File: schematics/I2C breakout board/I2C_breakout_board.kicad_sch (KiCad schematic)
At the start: 22 parts, among them J1 Conn_01x01_Pin, J10 Conn_01x01_Pin, J11 Conn_01x01_Pin, J12 Conn_01x01_Pin, J13 Conn_01x01_Pin, J14 Conn_01x01_Pin, J15 Conn_01x01_Pin, J16 Conn_01x01_Pin, J17 Conn_01x01_Pin, J2 Conn_01x01_Pin, J3 Conn_01x01_Pin, J4 Conn_01x01_Pin, J5 Conn_01x01_Pin, J6 Conn_01x01_Pin, J7 Conn_01x01_Pin, J8 Conn_01x01_Pin, J9 Conn_01x01_Pin, U1 ENS210-LQFM, U2 OPT4001DTSR

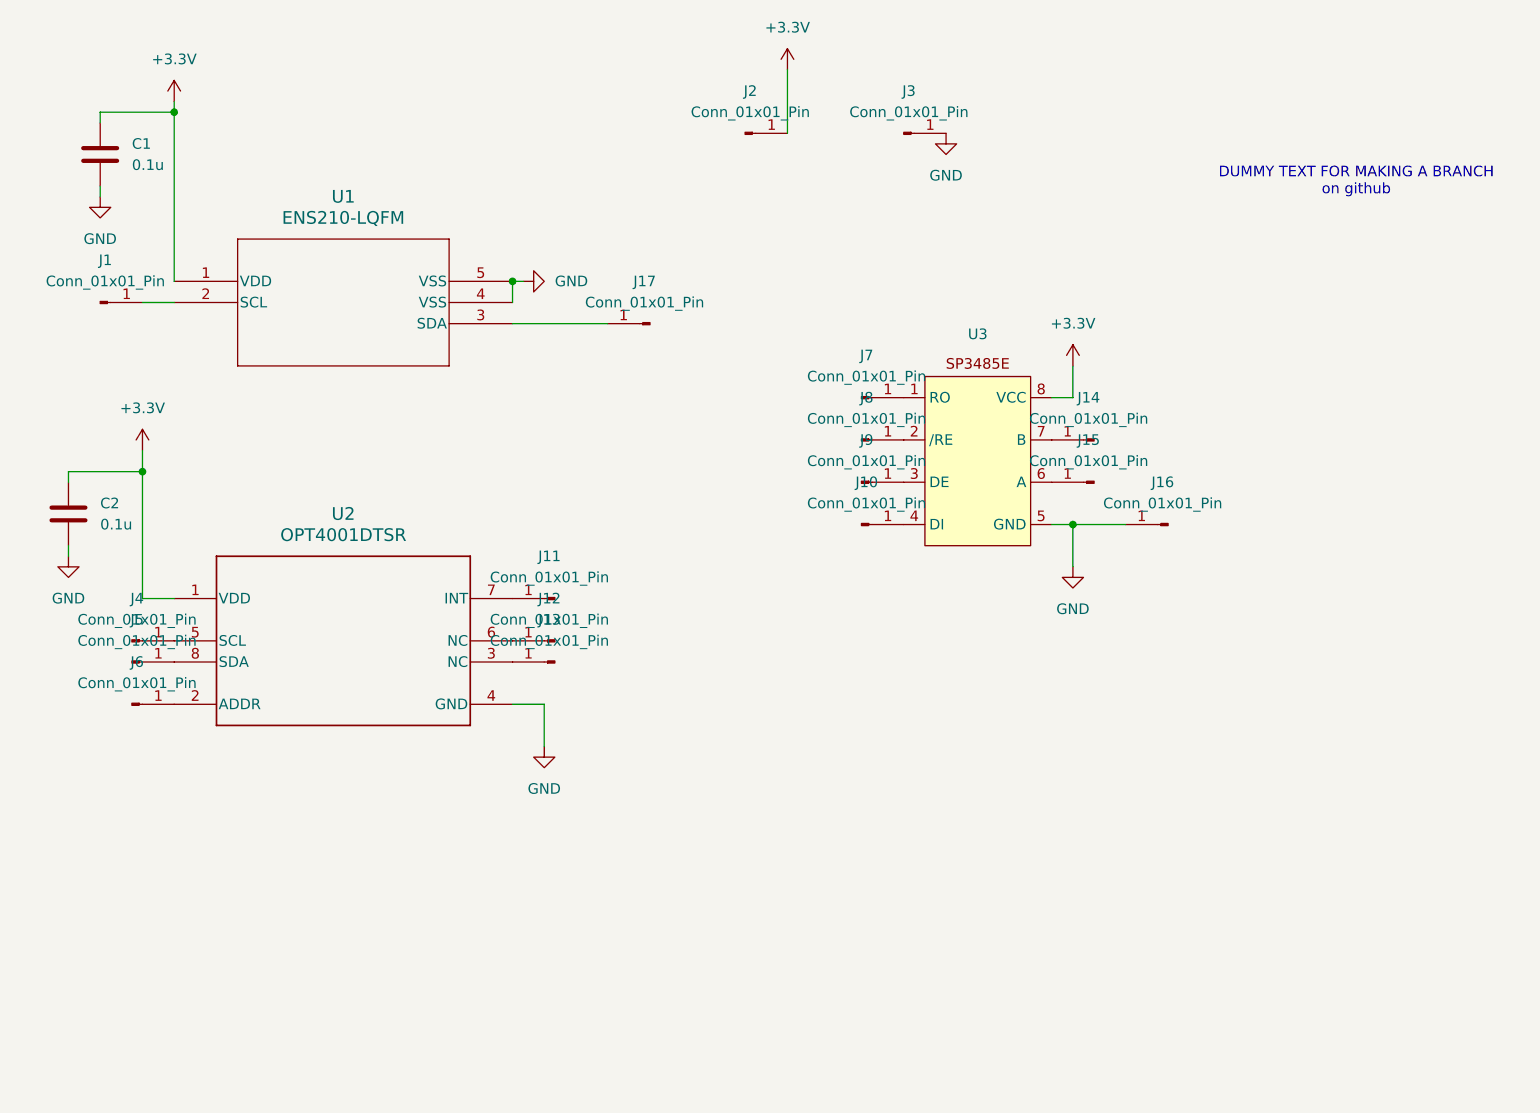
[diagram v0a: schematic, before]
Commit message: updated schematic
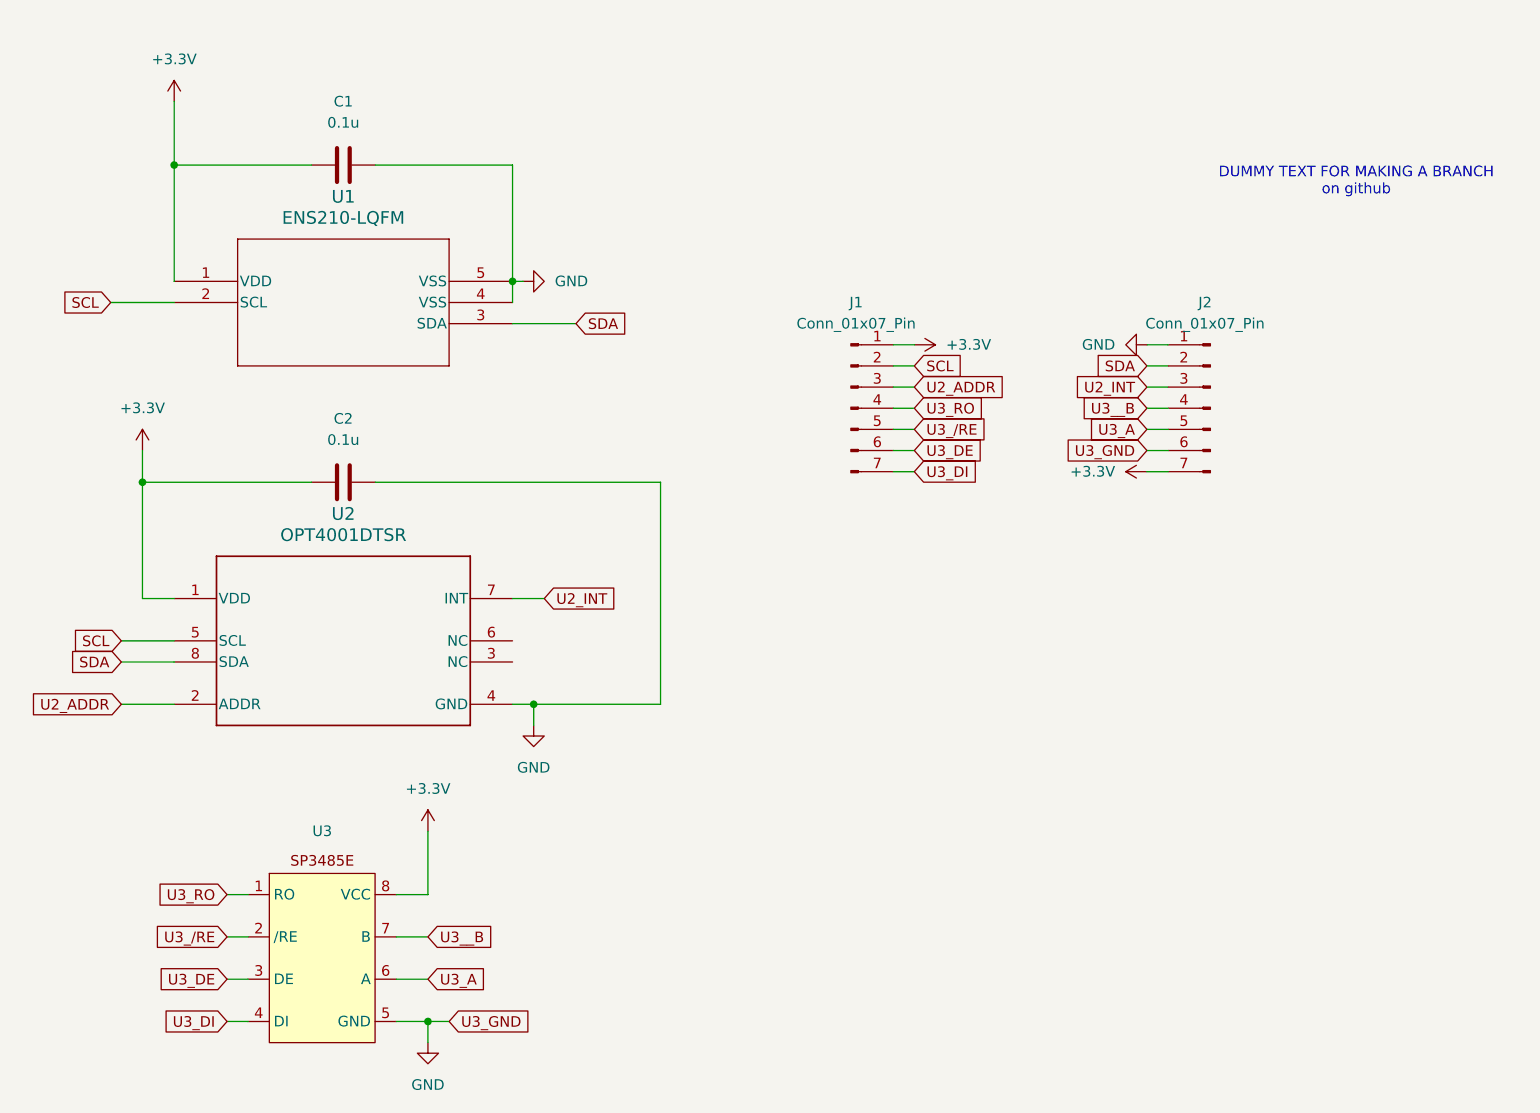
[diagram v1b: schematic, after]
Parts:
- removed J1, J10, J11, J12, J13, J14, J15, J16, J17, J2, J3, J4, J5, J6, J7, J8, J9: Conn_01x01_Pin, Connector_PinHeader_2.54mm:PinHeader_1x01_P2.54mm_Vertical, symbol Connector:Conn_01x01_Pin
- added J1, J2: Conn_01x07_Pin, Connector_PinHeader_2.54mm:PinHeader_1x07_P2.54mm_Vertical, symbol Connector:Conn_01x07_Pin
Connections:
- net +3.3V: now also J1.1 (Pin_1), J2.7 (Pin_7)
- net GND: now also J2.1 (Pin_1), J2.6 (Pin_6)
- net SCL: now reaches U1.2 (SCL)
- net SCL: now also U2.5 (SCL), J1.2 (Pin_2)
- net SDA: now reaches U1.3 (SDA)
- net SDA: now also U2.8 (SDA), J2.2 (Pin_2)
- net U3_DI: now reaches U3.4 (DI)
- net U3_DI: now also J1.7 (Pin_7)
- net U3_RO: now reaches U3.1 (RO)
- net U3_RO: now also J1.4 (Pin_4)
- net U2_ADDR: now reaches U2.2 (ADDR)
- net U2_ADDR: now also J1.3 (Pin_3)
- net U2_INT: now reaches U2.7 (INT)
- net U2_INT: now also J2.3 (Pin_3)
- net U3_DE: now reaches U3.3 (DE)
- net U3_DE: now also J1.6 (Pin_6)
- net U3_/RE: now reaches U3.2 (/RE)
- net U3_/RE: now also J1.5 (Pin_5)
- net U3__B: now reaches U3.7 (B)
- net U3__B: now also J2.4 (Pin_4)
- net U3_A: now reaches U3.6 (A)
- net U3_A: now also J2.5 (Pin_5)
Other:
- moved on the sheet: C1, C2

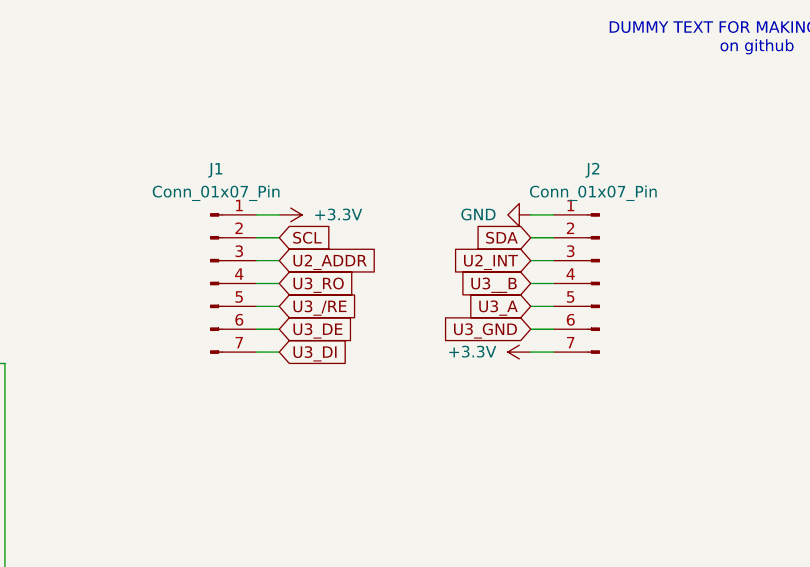
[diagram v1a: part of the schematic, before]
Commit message: finalized PCB for breakout board
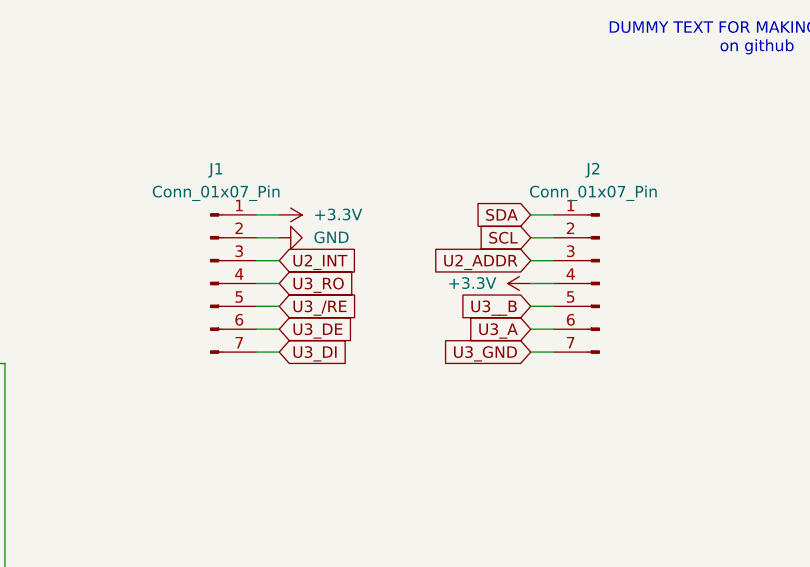
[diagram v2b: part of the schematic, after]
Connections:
- net +3.3V: now also J2.4 (Pin_4); no longer J2.7 (Pin_7)
- net GND: now also J1.2 (Pin_2), J2.7 (Pin_7); no longer J2.1 (Pin_1), J2.6 (Pin_6)
- net SCL: now also J2.2 (Pin_2); no longer J1.2 (Pin_2)
- net SDA: now also J2.1 (Pin_1); no longer J2.2 (Pin_2)
- net U2_ADDR: now also J2.3 (Pin_3); no longer J1.3 (Pin_3)
- net U2_INT: now also J1.3 (Pin_3); no longer J2.3 (Pin_3)
- net U3_A: now also J2.6 (Pin_6); no longer J2.5 (Pin_5)
- net U3__B: now also J2.5 (Pin_5); no longer J2.4 (Pin_4)
